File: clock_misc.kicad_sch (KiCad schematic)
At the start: 24 parts, among them J5 SWH, U19 74LVC1G06, U20 74LVC1G80, U21 FANOUT, Y1 TCXO

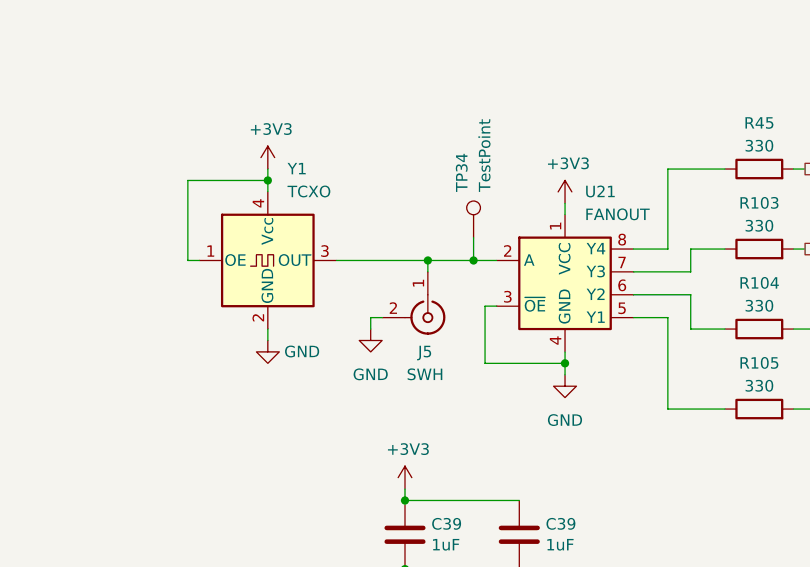
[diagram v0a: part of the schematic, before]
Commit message: add SWH connector symbols
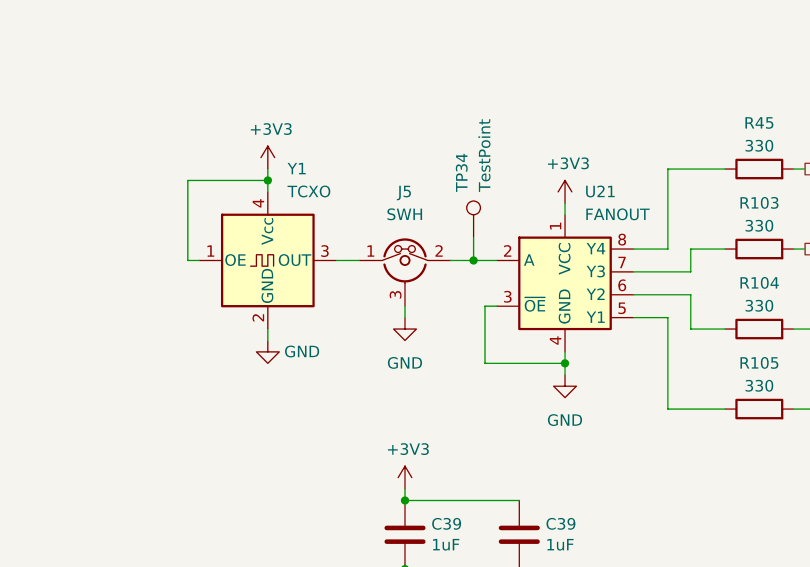
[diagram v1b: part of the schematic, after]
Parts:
- removed J5: SWH, symbol Connector:Conn_Coaxial
- added J5: SWH, symbol radio:Conn_Coaxial_MM8930-2620
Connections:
- net GND: now also J5.3 (Ext)
- net at TP34.1, U21.2 (A): now also J5.2 (R); no longer Y1.3 (OUT)
- new net: J5.1 (C), Y1.3 (OUT)
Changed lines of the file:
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@@
   (junction (at 173.99 123.19) (diameter 0) (color 0 0 0 0)
   )
-  (junction (at 78.74 76.2) (diameter 0) (color 0 0 0 0)
-  )
   (junction (at 40.64 168.91) (diameter 0) (color 0 0 0 0)
   )
@@
     (stroke (width 0) (type default))
   )
-  (wire (pts (xy 72.39 82.55) (xy 72.39 83.82))
+  (wire (pts (xy 76.2 81.28) (xy 76.2 82.55))
     (stroke (width 0) (type default))
   )
@@
     (stroke (width 0) (type default))
   )
-  (wire (pts (xy 78.74 76.2) (xy 83.82 76.2))
-    (stroke (width 0) (type default))
-  )
   (wire (pts (xy 60.96 67.31) (xy 60.96 68.58))
     (stroke (width 0) (type default))
@@
     (stroke (width 0) (type default))
   )
+  (wire (pts (xy 68.58 76.2) (xy 71.12 76.2))
+    (stroke (width 0) (type default))
+  )
   (wire (pts (xy 105.41 66.04) (xy 111.76 66.04))
     (stroke (width 0) (type default))
@@
     (stroke (width 0) (type default))
   )
+  (wire (pts (xy 81.28 76.2) (xy 83.82 76.2))
+    (stroke (width 0) (type default))
+  )
   (wire (pts (xy 119.38 74.93) (xy 120.65 74.93))
     (stroke (width 0) (type default))
@@
     (stroke (width 0) (type default))
   )
-  (wire (pts (xy 73.66 82.55) (xy 72.39 82.55))
-    (stroke (width 0) (type default))
-  )
   (wire (pts (xy 143.51 39.37) (xy 143.51 22.86))
     (stroke (width 0) (type default))
@@
     (stroke (width 0) (type default))
   )
-  (wire (pts (xy 68.58 76.2) (xy 78.74 76.2))
-    (stroke (width 0) (type default))
-  )
   (wire (pts (xy 171.45 39.37) (xy 170.18 39.37))
     (stroke (width 0) (type default))
@@
   )
   (wire (pts (xy 172.72 123.19) (xy 173.99 123.19))
-    (stroke (width 0) (type default))
-  )
-  (wire (pts (xy 78.74 76.2) (xy 78.74 77.47))
     (stroke (width 0) (type default))
   )
@@
     )
   )
-  (symbol (lib_id "Connector:Conn_Coaxial") (at 78.74 82.55 270) (unit 1)
-    (in_bom yes) (on_board yes) (dnp no) (fields_autoplaced)
-    (property "Reference" "J5" (at 78.4468 86.36 90)
-      (effects (font (size 1.27 1.27)))
-    )
-    (property "Value" "SWH" (at 78.4468 88.9 90)
-      (effects (font (size 1.27 1.27)))
-    )
-    (property "Footprint" "" (at 78.74 82.55 0)
-      (effects (font (size 1.27 1.27)) hide)
-    )
-    (property "Datasheet" " ~" (at 78.74 82.55 0)
-      (effects (font (size 1.27 1.27)) hide)
-    )
-    (property "Description" "COAX CONN TWO-WAY" (at 78.74 82.55 0)
-      (effects (font (size 1.27 1.27)) hide)
-    )
-    (property "Manufacturer" "Murata" (at 78.74 82.55 0)
-      (effects (font (size 1.27 1.27)) hide)
-    )
-    (property "Part Number" "MM8930-2620RJ4" (at 78.74 82.55 0)
-      (effects (font (size 1.27 1.27)) hide)
-    )
-    (property "Substitution" "MM8930-2620RK15" (at 78.74 82.55 0)
-      (effects (font (size 1.27 1.27)) hide)
-    )
-    (pin "1")
-    (pin "2")
-    (instances
-      (project "mainboard"
-        (path "/fb621148-8145-4217-9712-738e1b5a4823/4ec621be-184d-4855-a96d-f6fa2a788a77/90da2209-0e18-4bd4-8ef6-3d6f9ed46ff8"
-          (reference "J5") (unit 1)
-        )
-        (path "/fb621148-8145-4217-9712-738e1b5a4823/4ec621be-184d-4855-a96d-f6fa2a788a77/6aa278c8-8281-4438-81b7-90e6d7ac4f12"
-          (reference "J11") (unit 1)
-        )
-        (path "/fb621148-8145-4217-9712-738e1b5a4823/07741d92-cb3b-401f-9c7e-29f688af7269"
-          (reference "J12") (unit 1)
-        )
-      )
-    )
-  )
   (symbol (lib_id "support_hardware:3V3TX") (at 154.94 111.76 0) (unit 1)
     (in_bom yes) (on_board yes) (dnp no) (fields_autoplaced)
@@
     )
   )
+  (symbol (lib_id "radio:Conn_Coaxial_MM8930-2620") (at 76.2 76.2 0) (unit 1)
+    (in_bom yes) (on_board yes) (dnp no) (fields_autoplaced)
+    (property "Reference" "J5" (at 76.2 68.58 0)
+      (effects (font (size 1.27 1.27)))
+    )
+    (property "Value" "SWH" (at 76.2 71.12 0)
+      (effects (font (size 1.27 1.27)))
+    )
+    (property "Footprint" "" (at 76.2 76.2 0)
+      (effects (font (size 1.27 1.27)) hide)
+    )
+    (property "Datasheet" "https://www.murata.com/-/media/webrenewal/support/library/catalog/products/connector/o30e.ashx" (at 76.2 76.2 0)
+      (effects (font (size 1.27 1.27)) hide)
+    )
+    (property "Description" "COAX CONN TWO-WAY" (at 76.2 76.2 0)
+      (effects (font (size 1.27 1.27)) hide)
+    )
+    (property "Manufacturer" "Murata" (at 76.2 76.2 0)
+      (effects (font (size 1.27 1.27)) hide)
+    )
+    (property "Part Number" "MM8930-2620RJ4" (at 76.2 76.2 0)
+      (effects (font (size 1.27 1.27)) hide)
+    )
+    (property "Substitution" "MM8930-2620RK15" (at 76.2 76.2 0)
+      (effects (font (size 1.27 1.27)) hide)
+    )
+    (pin "2")
+    (pin "1")
+    (pin "3")
+    (instances
+      (project "mainboard"
+        (path "/fb621148-8145-4217-9712-738e1b5a4823/4ec621be-184d-4855-a96d-f6fa2a788a77/90da2209-0e18-4bd4-8ef6-3d6f9ed46ff8"
+          (reference "J5") (unit 1)
+        )
+        (path "/fb621148-8145-4217-9712-738e1b5a4823/07741d92-cb3b-401f-9c7e-29f688af7269"
+          (reference "J12") (unit 1)
+        )
+      )
+    )
+  )
   (symbol (lib_id "power:GND") (at 76.2 111.76 0) (unit 1)
     (in_bom yes) (on_board yes) (dnp no)
@@
     )
   )
-  (symbol (lib_id "power:GND") (at 72.39 83.82 0) (unit 1)
-    (in_bom yes) (on_board yes) (dnp no) (fields_autoplaced)
-    (property "Reference" "#PWR023" (at 72.39 90.17 0)
-      (effects (font (size 1.27 1.27)) hide)
-    )
-    (property "Value" "GND" (at 72.39 88.9 0)
-      (effects (font (size 1.27 1.27)))
-    )
-    (property "Footprint" "" (at 72.39 83.82 0)
-      (effects (font (size 1.27 1.27)) hide)
-    )
-    (property "Datasheet" "" (at 72.39 83.82 0)
-      (effects (font (size 1.27 1.27)) hide)
-    )
+  (symbol (lib_id "power:GND") (at 76.2 82.55 0) (unit 1)
+    (in_bom yes) (on_board yes) (dnp no) (fields_autoplaced)
+    (property "Reference" "#PWR023" (at 76.2 88.9 0)
+      (effects (font (size 1.27 1.27)) hide)
+    )
+    (property "Value" "GND" (at 76.2 87.63 0)
+      (effects (font (size 1.27 1.27)))
+    )
+    (property "Footprint" "" (at 76.2 82.55 0)
+      (effects (font (size 1.27 1.27)) hide)
+    )
+    (property "Datasheet" "" (at 76.2 82.55 0)
+      (effects (font (size 1.27 1.27)) hide)
+    )
